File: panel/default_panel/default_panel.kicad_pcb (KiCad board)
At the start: 2 copper layers, 100 x 100 mm, 1 part

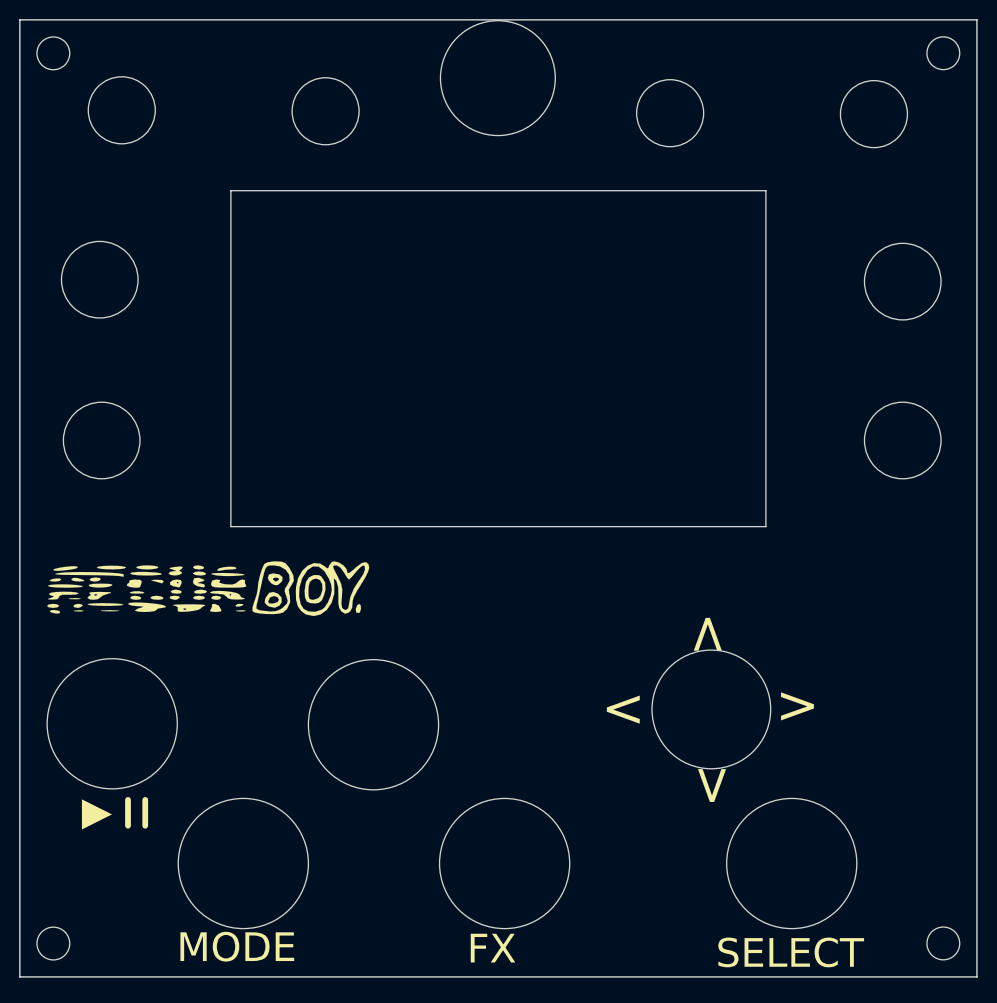
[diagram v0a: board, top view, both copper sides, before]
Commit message: some panel stuff
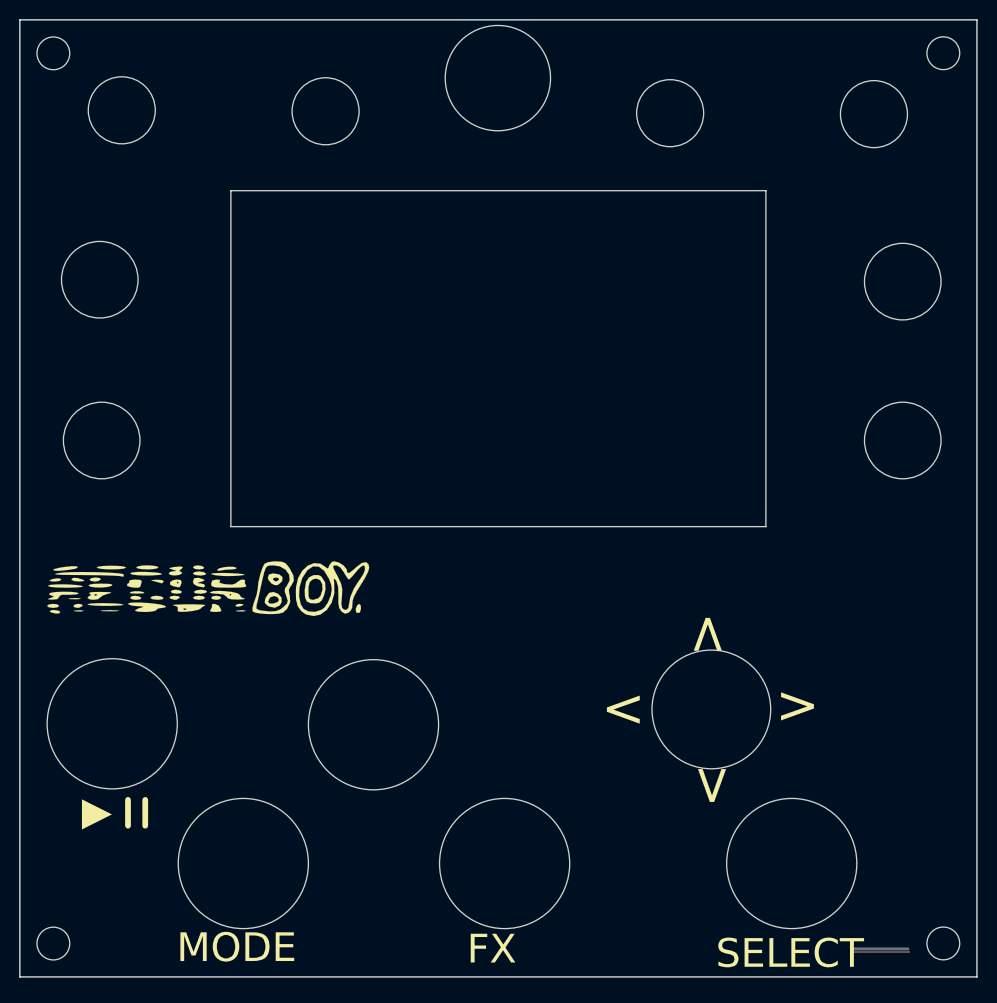
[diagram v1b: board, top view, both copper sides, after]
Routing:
- net (no net): track 0.00 -> 12.0 mm
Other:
- outline, holes or cut-outs redrawn
